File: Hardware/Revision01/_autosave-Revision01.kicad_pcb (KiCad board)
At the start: 2 copper layers, 67 parts, among them Q3 NMOS, Q4 PMOS, Q6 PMOS, U1 NUCLEO-L476RG, U10 NCP1117LPST50T3G, U2 MRF89XAM9AT-I/RM, U4 ICM-45605

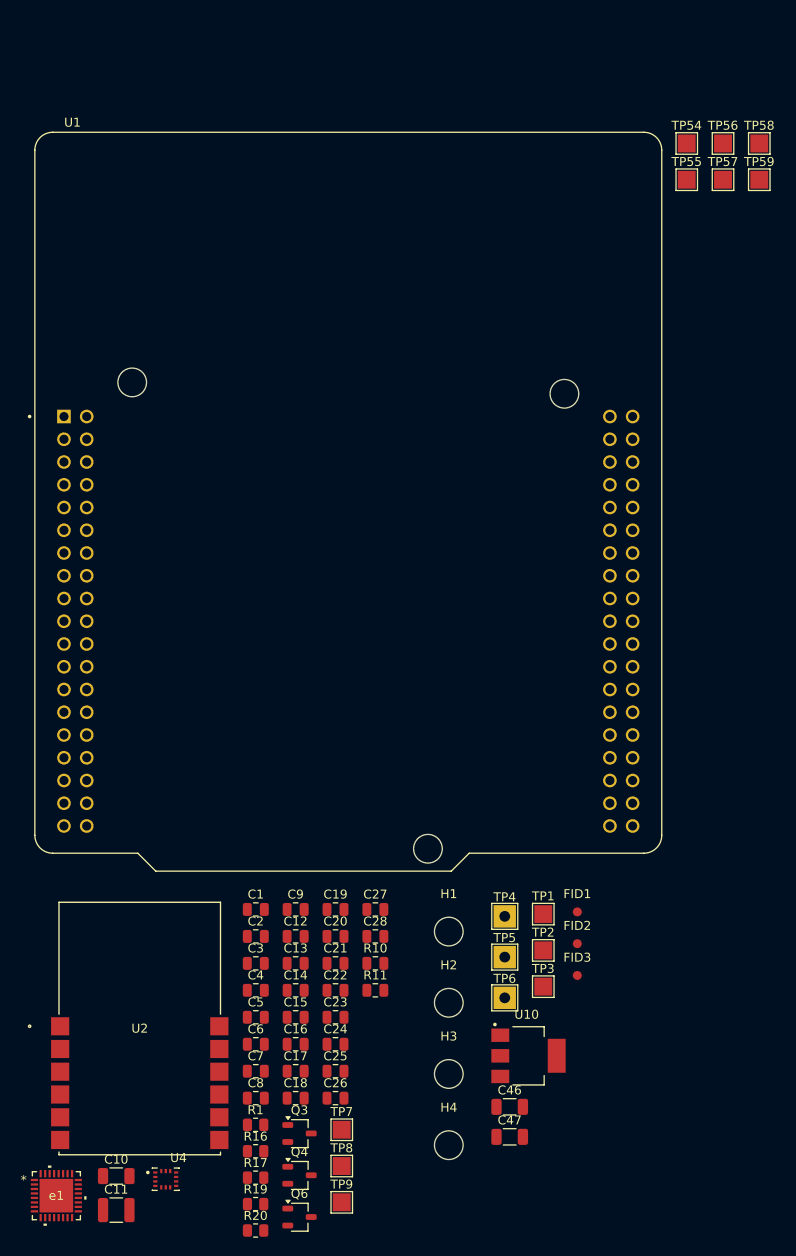
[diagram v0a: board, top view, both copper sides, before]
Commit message: starting to work on LAYOUT
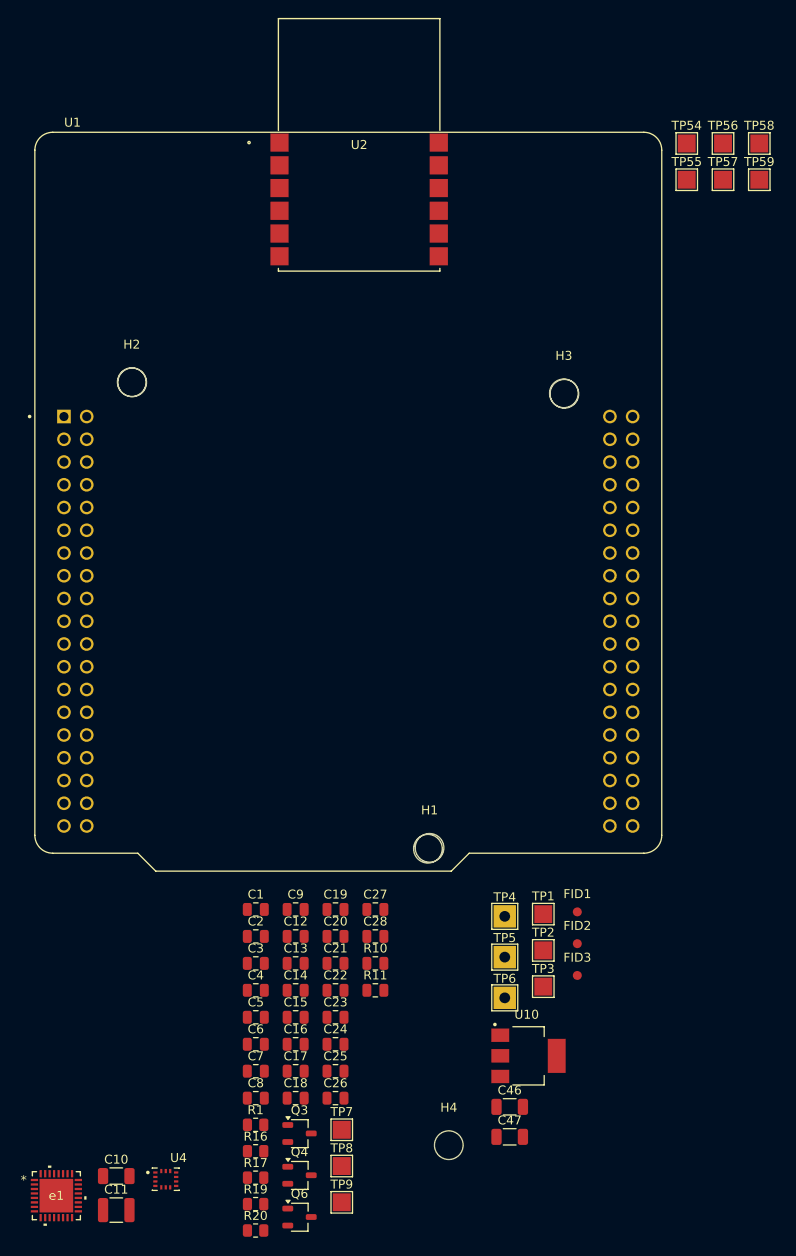
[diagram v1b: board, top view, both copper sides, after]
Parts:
- moved U2 101.7 mm to (143.1, 54.8)
- moved H2 77.8 mm to (117.8, 81.2)
- moved H3 77.1 mm to (166.0, 82.5)
- moved H1 9.59 mm to (151.0, 133.2)
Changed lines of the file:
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@@
 	(footprint "MountingHole:MountingHole_3.2mm_M3"
 		(layer "F.Cu")
-		(at 153.15 150.55)
+		(at 117.75 81.25)
 		(descr "Mounting Hole 3.2mm, no annular, M3")
 		(tags "mounting hole 3.2mm no annular m3")
@@
 	(footprint "MRF89XAM9AT-antenna:MOD_MRF89XAM9A_MCH"
 		(layer "F.Cu")
-		(at 118.6418 153.4252)
+		(at 143.14 54.754)
 		(tags "MRF89XAM9AT-I/RM ")
 		(property "Reference" "U2"
@@
 	(footprint "MountingHole:MountingHole_3.2mm_M3"
 		(layer "F.Cu")
-		(at 153.15 158.5)
+		(at 166 82.5)
 		(descr "Mounting Hole 3.2mm, no annular, M3")
 		(tags "mounting hole 3.2mm no annular m3")
@@
 	(footprint "MountingHole:MountingHole_3.2mm_M3"
 		(layer "F.Cu")
-		(at 153.15 142.6)
+		(at 151 133.25)
 		(descr "Mounting Hole 3.2mm, no annular, M3")
 		(tags "mounting hole 3.2mm no annular m3")
